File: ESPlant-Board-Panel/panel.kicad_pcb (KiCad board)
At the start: 2 copper layers, 156 x 147 mm, 408 parts, among them J1 Conn_01x05, U1 ESP32-C6-MINI-1/U, U3 Reset, U4 Boot, U5 Temp/Humid-Sensor, U6 Light sensor, U7 AMS1117-3_3, U8 MK-12C02-G025

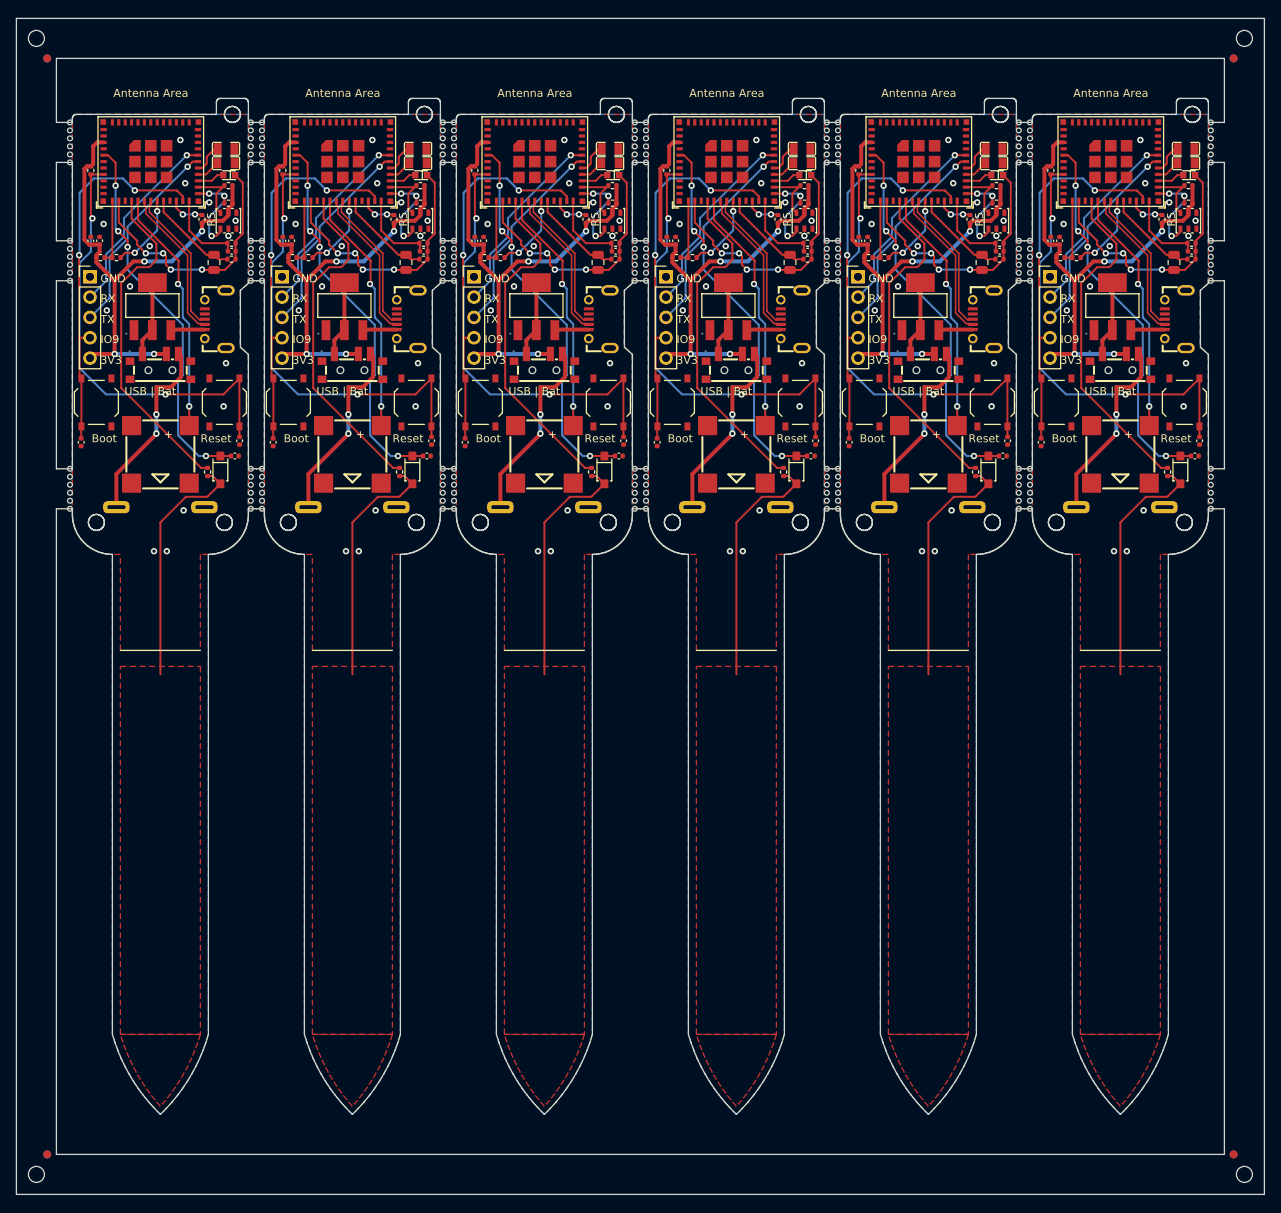
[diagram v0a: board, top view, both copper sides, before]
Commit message: Finish v2.0 for prototyping
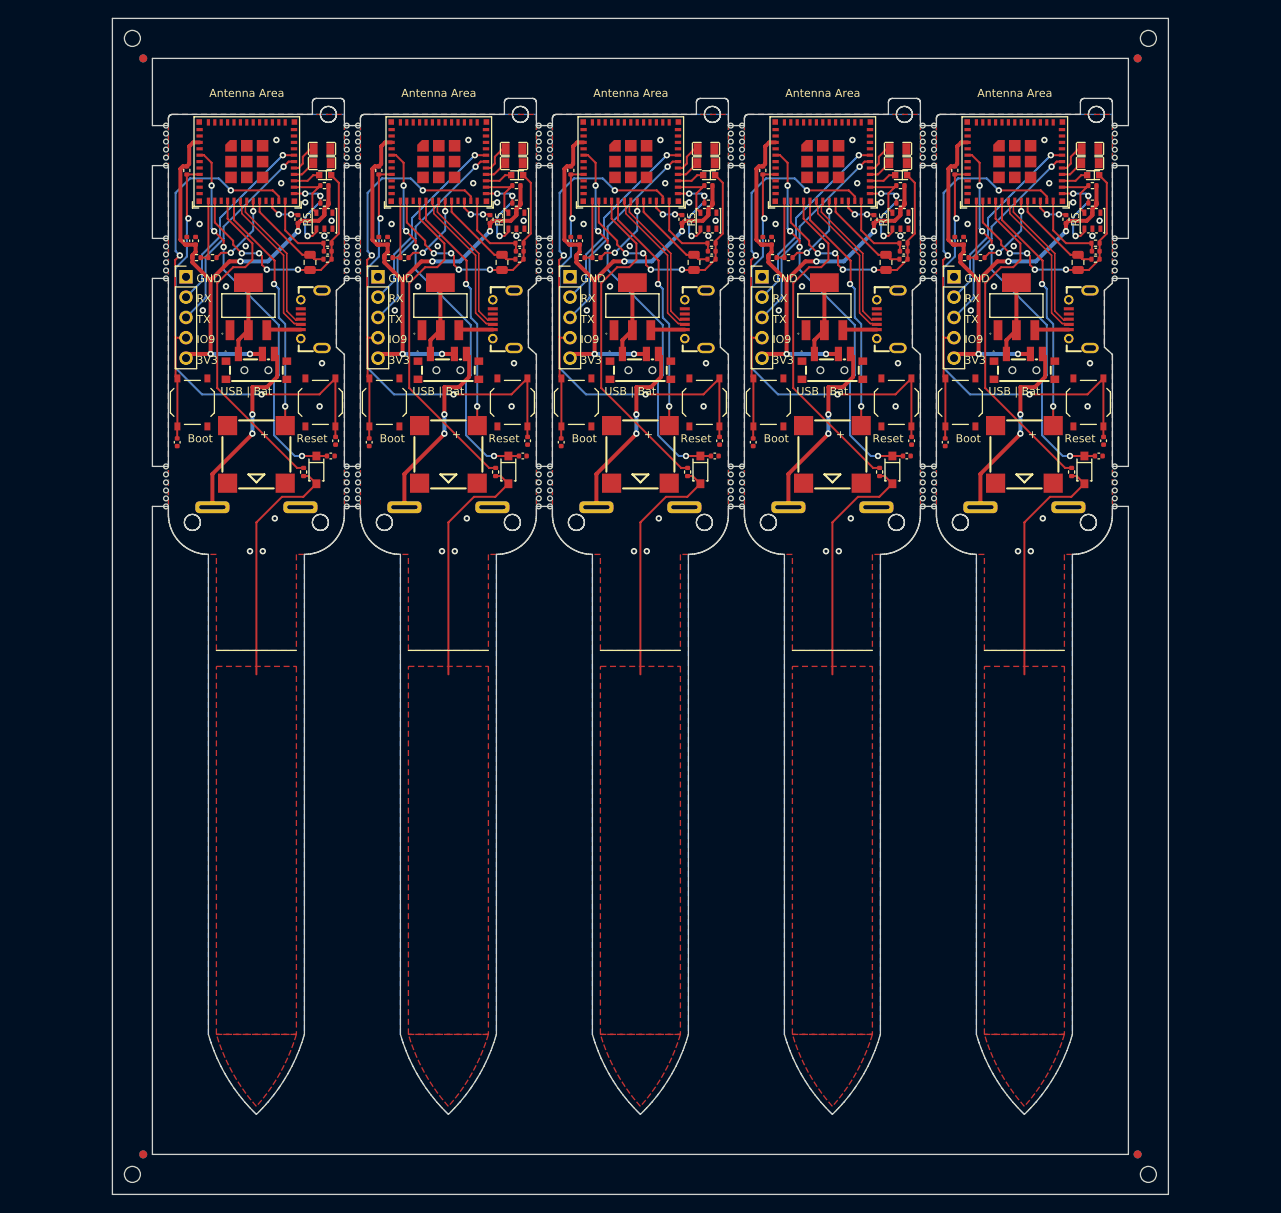
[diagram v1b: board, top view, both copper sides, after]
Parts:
- removed the BZ1 at (165.0, 74.5)
- removed the BZ1 at (237.0, 74.5)
- removed the BZ1 at (189.0, 74.5)
- removed the BZ1 at (213.0, 74.5)
- removed the BZ1 at (285.0, 74.5)
- removed the BZ1 at (261.0, 74.5)
- removed the C1 at (270.9, 72.8)
- removed the C1 at (198.9, 72.8)
- removed the C1 at (222.9, 72.8)
- removed the C1 at (246.9, 72.8)
- removed the C1 at (294.9, 72.8)
- removed the C1 at (174.9, 72.8)
- removed the C2 at (155.1, 73.0)
- removed the C2 at (251.1, 73.0)
- removed the C2 at (179.1, 73.0)
- removed the C2 at (275.1, 73.0)
- removed the C2 at (227.1, 73.0)
- removed the C2 at (203.1, 73.0)
- removed the C3 at (294.3, 74.7)
- removed the C3 at (222.3, 74.7)
- removed the C3 at (198.3, 74.7)
- removed the C3 at (246.3, 74.7)
- removed the C3 at (174.3, 74.7)
- removed the C3 at (270.3, 74.7)
- removed the C5 at (173.9, 49.1)
- removed the C5 at (269.9, 49.1)
- removed the C5 at (197.9, 49.1)
- removed the C5 at (293.9, 49.1)
- removed the C5 at (221.9, 49.1)
- removed the C5 at (245.9, 49.1)
- removed the C7 at (243.7, 50.5)
- removed the C7 at (219.7, 50.5)
- removed the C7 at (195.7, 50.5)
- removed the C7 at (267.7, 50.5)
- removed the C7 at (171.7, 50.5)
- removed the C7 at (291.7, 50.5)
- removed the C8 at (181.4, 47.8)
- removed the C8 at (229.4, 47.8)
- removed the C8 at (205.4, 47.8)
- removed the C8 at (253.4, 47.8)
- removed the C8 at (157.4, 47.8)
- removed the C8 at (277.4, 47.8)
- removed the C9 at (252.3, 47.8)
- removed the C9 at (204.3, 47.8)
- removed the C9 at (228.3, 47.8)
- removed the C9 at (156.3, 47.8)
- removed the C9 at (276.3, 47.8)
- removed the C9 at (180.3, 47.8)
- removed the D1 at (245.2, 36.3)
- removed the D1 at (293.2, 36.3)
- removed the D1 at (269.2, 36.3)
- removed the D1 at (221.2, 36.3)
- removed the D1 at (173.2, 36.3)
- removed the D1 at (197.2, 36.3)
- removed the D2 at (172.5, 76.4)
- removed the D2 at (220.5, 76.4)
- removed the D2 at (196.5, 76.4)
- removed the D2 at (292.5, 76.4)
- removed the D2 at (268.5, 76.4)
- removed the D2 at (244.5, 76.4)
- removed the D3 at (173.2, 38.1)
- removed the D3 at (197.2, 38.1)
- removed the D3 at (221.2, 38.1)
- removed the D3 at (245.2, 38.1)
- removed the D3 at (269.2, 38.1)
- removed the D3 at (293.2, 38.1)
- removed the J1 at (276.2, 52.3)
- removed the J1 at (204.2, 52.3)
- removed the J1 at (180.2, 52.3)
- removed the J1 at (228.2, 52.3)
- removed the J1 at (252.2, 52.3)
- removed the J1 at (156.2, 52.3)
- removed the R1 at (269.9, 48.1)
- removed the R1 at (173.9, 48.1)
- removed the R1 at (293.9, 48.1)
- removed the R1 at (221.9, 48.1)
- removed the R1 at (245.9, 48.1)
- removed the R1 at (197.9, 48.1)
- removed the R10 at (221.5, 43.1)
- removed the R10 at (245.5, 43.1)
- removed the R10 at (293.5, 43.1)
- removed the R10 at (197.5, 43.1)
- removed the R10 at (173.5, 43.1)
- removed the R10 at (269.5, 43.1)
- removed the R2 at (245.5, 40.9)
- removed the R2 at (221.5, 40.9)
- removed the R2 at (269.5, 40.9)
- removed the R2 at (293.5, 40.9)
- removed the R2 at (173.5, 40.9)
- removed the R2 at (197.5, 40.9)
- removed the R3 at (197.9, 50.1)
- removed the R3 at (173.9, 50.1)
- removed the R3 at (293.9, 50.1)
- removed the R3 at (245.9, 50.1)
- removed the R3 at (221.9, 50.1)
- removed the R3 at (269.9, 50.1)
- removed the R4 at (277.5, 49.9)
- removed the R4 at (205.5, 49.9)
- removed the R4 at (157.5, 49.9)
- removed the R4 at (181.5, 49.9)
- removed the R4 at (253.5, 49.9)
- removed the R4 at (229.5, 49.9)
- removed the R5 at (170.2, 45.1)
- removed the R5 at (266.2, 45.1)
- removed the R5 at (242.2, 45.1)
- removed the R5 at (194.2, 45.1)
- removed the R5 at (290.2, 45.1)
- removed the R5 at (218.2, 45.1)
- removed the R6 at (231.5, 49.9)
- removed the R6 at (183.5, 49.9)
- removed the R6 at (207.5, 49.9)
- removed the R6 at (255.5, 49.9)
- removed the R6 at (279.5, 49.9)
- removed the R6 at (159.5, 49.9)
- removed the R8 at (194.9, 76.7)
- removed the R8 at (266.9, 76.7)
- removed the R8 at (242.9, 76.7)
- removed the R8 at (290.9, 76.7)
- removed the R8 at (218.9, 76.7)
- removed the R8 at (170.9, 76.7)
- removed the R9 at (180.3, 39.0)
- removed the R9 at (252.3, 39.0)
- removed the R9 at (276.3, 39.0)
- removed the R9 at (204.3, 39.0)
- removed the R9 at (228.3, 39.0)
- removed the R9 at (156.3, 39.0)
- removed the REF** at (296.3, 34.0)
- removed the REF** at (224.3, 79.3)
- removed the REF** at (201.7, 50.8)
- removed the REF** at (249.7, 79.3)
- removed the REF** at (201.7, 79.3)
- removed the REF** at (200.3, 80.3)
- removed the REF** at (224.3, 51.8)
- removed the REF** at (153.7, 33.0)
- removed the REF** at (225.7, 50.8)
- removed the REF** at (200.3, 34.0)
- removed the REF** at (201.7, 52.8)
- removed the REF** at (176.3, 35.0)
- removed the REF** at (300.5, 164.5)
- removed the REF** at (201.7, 47.8)
- removed the REF** at (224.3, 50.8)
- removed the REF** at (272.3, 52.8)
- removed the REF** at (248.3, 48.8)
- removed the REF** at (248.3, 50.8)
- removed the REF** at (248.3, 36.0)
- removed the REF** at (176.3, 36.0)
- removed the REF** at (296.3, 52.8)
- removed the REF** at (273.7, 80.3)
- removed the REF** at (153.7, 80.3)
- removed the REF** at (225.7, 38.0)
- removed the REF** at (249.7, 36.0)
- removed the REF** at (177.7, 36.0)
- removed the REF** at (150.9, 25.0) (x2)
- removed the REF** at (177.7, 81.3)
- removed the REF** at (249.7, 48.8)
- removed the REF** at (224.3, 33.0)
- removed the REF** at (153.7, 35.0)
- removed the REF** at (272.3, 35.0)
- removed the REF** at (201.7, 36.0)
- removed the REF** at (225.7, 78.3)
- removed the REF** at (272.3, 38.0)
- removed the REF** at (224.3, 34.0)
- removed the REF** at (153.7, 52.8)
- removed the REF** at (200.3, 77.3)
- removed the REF** at (177.7, 76.3)
- removed the REF** at (201.7, 80.3)
- removed the REF** at (224.3, 35.0)
- removed the REF** at (225.7, 76.3)
- removed the REF** at (225.7, 79.3)
- removed the REF** at (225.7, 77.3)
- removed the REF** at (225.7, 48.8)
- removed the REF** at (150.9, 162.0) (x2)
- removed the REF** at (272.3, 49.8)
- removed the REF** at (296.3, 81.3)
- removed the REF** at (248.3, 79.3)
- removed the REF** at (299.2, 162.0) (x2)
- removed the REF** at (249.7, 34.0)
- removed the REF** at (200.3, 49.8)
- removed the REF** at (273.7, 47.8)
- removed the REF** at (200.3, 38.0)
- removed the REF** at (200.3, 52.8)
- removed the REF** at (272.3, 48.8)
- removed the REF** at (176.3, 79.3)
- removed the REF** at (149.5, 164.5)
- removed the REF** at (273.7, 37.0)
- removed the REF** at (273.7, 81.3)
- removed the REF** at (225.7, 34.0)
- removed the REF** at (248.3, 78.3)
- removed the REF** at (249.7, 37.0)
- removed the REF** at (153.7, 76.3)
- removed the REF** at (201.7, 35.0)
- removed the REF** at (153.7, 47.8)
- removed the REF** at (296.3, 38.0)
- removed the REF** at (296.3, 78.3)
- removed the REF** at (176.3, 33.0)
- removed the REF** at (176.3, 37.0)
- removed the REF** at (248.3, 49.8)
- removed the REF** at (249.7, 50.8)
- removed the REF** at (272.3, 76.3)
- removed the REF** at (200.3, 36.0)
- removed the REF** at (273.7, 33.0)
- removed the REF** at (273.7, 78.3)
- removed the REF** at (248.3, 81.3)
- removed the REF** at (248.3, 35.0)
- removed the REF** at (224.3, 49.8)
- removed the REF** at (225.7, 36.0)
- removed the REF** at (296.3, 47.8)
- removed the REF** at (153.7, 81.3)
- removed the REF** at (176.3, 38.0)
- removed the REF** at (177.7, 34.0)
- removed the REF** at (249.7, 47.8)
- removed the REF** at (225.7, 47.8)
- removed the REF** at (153.7, 34.0)
- removed the REF** at (177.7, 37.0)
- removed the REF** at (200.3, 48.8)
- removed the REF** at (225.7, 52.8)
- removed the REF** at (296.3, 49.8)
- removed the REF** at (248.3, 37.0)
- removed the REF** at (296.3, 76.3)
- removed the REF** at (273.7, 35.0)
- removed the REF** at (201.7, 38.0)
- removed the REF** at (201.7, 48.8)
- removed the REF** at (248.3, 38.0)
- removed the REF** at (176.3, 77.3)
- removed the REF** at (224.3, 78.3)
- removed the REF** at (177.7, 35.0)
- removed the REF** at (224.3, 47.8)
- removed the REF** at (176.3, 51.8)
- removed the REF** at (273.7, 52.8)
- removed the REF** at (153.7, 50.8)
- removed the REF** at (248.3, 47.8)
- removed the REF** at (201.7, 51.8)
- removed the REF** at (272.3, 80.3)
- removed the REF** at (153.7, 48.8)
- removed the REF** at (153.7, 38.0)
- removed the REF** at (299.2, 25.0) (x2)
- removed the REF** at (296.3, 80.3)
- removed the REF** at (225.7, 33.0)
- removed the REF** at (273.7, 34.0)
- removed the REF** at (177.7, 50.8)
- removed the REF** at (176.3, 50.8)
- removed the REF** at (273.7, 36.0)
- removed the REF** at (153.7, 36.0)
- removed the REF** at (249.7, 80.3)
- removed the REF** at (176.3, 48.8)
- removed the REF** at (200.3, 76.3)
- removed the REF** at (273.7, 79.3)
- removed the REF** at (248.3, 80.3)
- removed the REF** at (153.7, 79.3)
- removed the REF** at (176.3, 78.3)
- removed the REF** at (296.3, 77.3)
- removed the REF** at (249.7, 76.3)
- removed the REF** at (177.7, 47.8)
- removed the REF** at (177.7, 33.0)
- removed the REF** at (224.3, 37.0)
- removed the REF** at (248.3, 33.0)
- removed the REF** at (200.3, 78.3)
- removed the REF** at (272.3, 81.3)
- removed the REF** at (296.3, 50.8)
- removed the REF** at (153.7, 37.0)
- removed the REF** at (225.7, 49.8)
- removed the REF** at (248.3, 34.0)
- removed the REF** at (225.7, 51.8)
- removed the REF** at (272.3, 77.3)
- removed the REF** at (248.3, 52.8)
- removed the REF** at (201.7, 76.3)
- removed the REF** at (177.7, 80.3)
- removed the REF** at (201.7, 81.3)
- removed the REF** at (153.7, 51.8)
- removed the REF** at (296.3, 48.8)
- removed the REF** at (149.5, 22.5)
- removed the REF** at (177.7, 49.8)
- removed the REF** at (200.3, 35.0)
- removed the REF** at (273.7, 76.3)
- removed the REF** at (201.7, 49.8)
- removed the REF** at (249.7, 77.3)
- removed the REF** at (272.3, 37.0)
- removed the REF** at (249.7, 35.0)
- removed the REF** at (248.3, 77.3)
- removed the REF** at (201.7, 37.0)
- removed the REF** at (273.7, 50.8)
- removed the REF** at (177.7, 52.8)
- removed the REF** at (249.7, 78.3)
- removed the REF** at (296.3, 79.3)
- removed the REF** at (224.3, 36.0)
- removed the REF** at (153.7, 78.3)
- removed the REF** at (296.3, 51.8)
- removed the REF** at (249.7, 49.8)
- removed the REF** at (200.3, 79.3)
- removed the REF** at (176.3, 34.0)
- removed the REF** at (201.7, 33.0)
- removed the REF** at (248.3, 51.8)
- removed the REF** at (224.3, 48.8)
- removed the REF** at (272.3, 51.8)
- removed the REF** at (296.3, 33.0)
- removed the REF** at (177.7, 77.3)
- removed the REF** at (272.3, 78.3)
- removed the REF** at (200.3, 33.0)
- removed the REF** at (300.5, 22.5)
- removed the REF** at (176.3, 81.3)
- removed the REF** at (225.7, 35.0)
- removed the REF** at (225.7, 80.3)
- removed the REF** at (224.3, 81.3)
- removed the REF** at (224.3, 77.3)
- removed the REF** at (153.7, 77.3)
- removed the REF** at (177.7, 78.3)
- removed the REF** at (177.7, 51.8)
- removed the REF** at (272.3, 36.0)
- removed the REF** at (249.7, 38.0)
- removed the REF** at (225.7, 37.0)
- removed the REF** at (200.3, 81.3)
- removed the REF** at (296.3, 35.0)
- removed the REF** at (200.3, 51.8)
- removed the REF** at (176.3, 80.3)
- removed the REF** at (201.7, 34.0)
- removed the REF** at (249.7, 81.3)
- removed the REF** at (272.3, 33.0)
- removed the REF** at (272.3, 79.3)
- removed the REF** at (273.7, 77.3)
- removed the REF** at (272.3, 34.0)
- removed the REF** at (224.3, 76.3)
- removed the REF** at (176.3, 76.3)
- removed the REF** at (201.7, 77.3)
- removed the REF** at (176.3, 47.8)
- removed the REF** at (272.3, 47.8)
- removed the REF** at (224.3, 80.3)
- removed the REF** at (177.7, 38.0)
- removed the REF** at (249.7, 52.8)
- removed the REF** at (177.7, 79.3)
- removed the REF** at (200.3, 47.8)
- removed the REF** at (224.3, 38.0)
- removed the REF** at (273.7, 38.0)
- removed the REF** at (249.7, 33.0)
- removed the REF** at (296.3, 37.0)
- removed the REF** at (224.3, 52.8)
- removed the REF** at (273.7, 49.8)
- removed the REF** at (200.3, 50.8)
- removed the REF** at (177.7, 48.8)
- removed the REF** at (176.3, 52.8)
- removed the REF** at (200.3, 37.0)
- removed the REF** at (273.7, 51.8)
- removed the REF** at (225.7, 81.3)
- removed the REF** at (201.7, 78.3)
- removed the REF** at (273.7, 48.8)
- removed the REF** at (176.3, 49.8)
- removed the REF** at (296.3, 36.0)
- removed the REF** at (153.7, 49.8)
- removed the REF** at (272.3, 50.8)
- removed the REF** at (249.7, 51.8)
- removed the REF** at (248.3, 76.3)
- removed the U1 at (211.8, 35.2)
- removed the U1 at (235.8, 35.2)
- removed the U1 at (259.8, 35.2)
- removed the U1 at (283.8, 35.2)
- removed the U1 at (187.8, 35.2)
- removed the U1 at (163.8, 35.2)
- removed the U3 at (269.0, 68.0)
- removed the U3 at (221.0, 68.0)
- removed the U3 at (245.0, 68.0)
- removed the U3 at (293.0, 68.0)
- removed the U3 at (173.0, 68.0)
- removed the U3 at (197.0, 68.0)
- removed the U4 at (181.0, 68.0)
- removed the U4 at (229.0, 68.0)
- removed the U4 at (277.0, 68.0)
- removed the U4 at (205.0, 68.0)
- removed the U4 at (157.0, 68.0)
- removed the U4 at (253.0, 68.0)
- removed the U5 at (269.5, 45.3)
- removed the U5 at (293.5, 45.3)
- removed the U5 at (173.5, 45.3)
- removed the U5 at (221.5, 45.3)
- removed the U5 at (245.5, 45.3)
- removed the U5 at (197.5, 45.3)
- removed the U6 at (245.6, 39.6)
- removed the U6 at (221.6, 39.6)
- removed the U6 at (173.6, 39.6)
- removed the U6 at (293.6, 39.6)
- removed the U6 at (269.6, 39.6)
- removed the U6 at (197.6, 39.6)
- removed the U7 at (188.0, 56.0)
- removed the U7 at (164.0, 56.0)
- removed the U7 at (236.0, 56.0)
- removed the U7 at (212.0, 56.0)
- removed the U7 at (260.0, 56.0)
- removed the U7 at (284.0, 56.0)
- removed the U8 at (285.0, 63.5)
- removed the U8 at (237.0, 63.5)
- removed the U8 at (261.0, 63.5)
- removed the U8 at (165.0, 63.5)
- removed the U8 at (213.0, 63.5)
- removed the U8 at (189.0, 63.5)
- removed the U9 at (165.0, 81.1)
- removed the U9 at (285.0, 81.1)
- removed the U9 at (213.0, 81.1)
- removed the U9 at (261.0, 81.1)
- removed the U9 at (189.0, 81.1)
- removed the U9 at (237.0, 81.1)
- removed the USB1 at (195.9, 57.6)
- removed the USB1 at (267.9, 57.6)
- removed the USB1 at (219.9, 57.6)
- removed the USB1 at (171.9, 57.6)
- removed the USB1 at (243.9, 57.6)
- removed the USB1 at (291.9, 57.6)
- added BZ1: Buzzer, CustomFootprints:BUZ-SMD_4P-L8.5-W8.5-P8.50-BR, F.Cu at (249.0, 74.5)
- added BZ1: Buzzer, CustomFootprints:BUZ-SMD_4P-L8.5-W8.5-P8.50-BR, F.Cu at (201.0, 74.5)
- added BZ1: Buzzer, CustomFootprints:BUZ-SMD_4P-L8.5-W8.5-P8.50-BR, F.Cu at (177.0, 74.5)
- added BZ1: Buzzer, CustomFootprints:BUZ-SMD_4P-L8.5-W8.5-P8.50-BR, F.Cu at (273.0, 74.5)
- added BZ1: Buzzer, CustomFootprints:BUZ-SMD_4P-L8.5-W8.5-P8.50-BR, F.Cu at (225.0, 74.5)
- added C1: 100nF, Capacitor_SMD:C_0402_1005Metric, F.Cu at (186.9, 72.8)
- added C1: 100nF, Capacitor_SMD:C_0402_1005Metric, F.Cu at (210.9, 72.8)
- added C1: 100nF, Capacitor_SMD:C_0402_1005Metric, F.Cu at (258.9, 72.8)
- added C1: 100nF, Capacitor_SMD:C_0402_1005Metric, F.Cu at (234.9, 72.8)
- added C1: 100nF, Capacitor_SMD:C_0402_1005Metric, F.Cu at (282.9, 72.8)
- added C2: 100nF, Capacitor_SMD:C_0402_1005Metric, F.Cu at (263.1, 73.0)
- added C2: 100nF, Capacitor_SMD:C_0402_1005Metric, F.Cu at (239.1, 73.0)
- added C2: 100nF, Capacitor_SMD:C_0402_1005Metric, F.Cu at (215.1, 73.0)
- added C2: 100nF, Capacitor_SMD:C_0402_1005Metric, F.Cu at (167.1, 73.0)
- added C2: 100nF, Capacitor_SMD:C_0402_1005Metric, F.Cu at (191.1, 73.0)
- added C3: 150pF, Capacitor_SMD:C_0402_1005Metric, F.Cu at (210.3, 74.7)
- added C3: 150pF, Capacitor_SMD:C_0402_1005Metric, F.Cu at (258.3, 74.7)
- added C3: 150pF, Capacitor_SMD:C_0402_1005Metric, F.Cu at (186.3, 74.7)
- added C3: 150pF, Capacitor_SMD:C_0402_1005Metric, F.Cu at (234.3, 74.7)
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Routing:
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- removed copper zone on F.Cu, net Board_5-/SensorCapV
- removed copper zone on B.Cu, net Board_5-GND
- removed copper zone on F.Cu, net Board_5-GND
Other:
- board size 156 x 147 mm -> 132 x 147 mm

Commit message: Board: Update panel
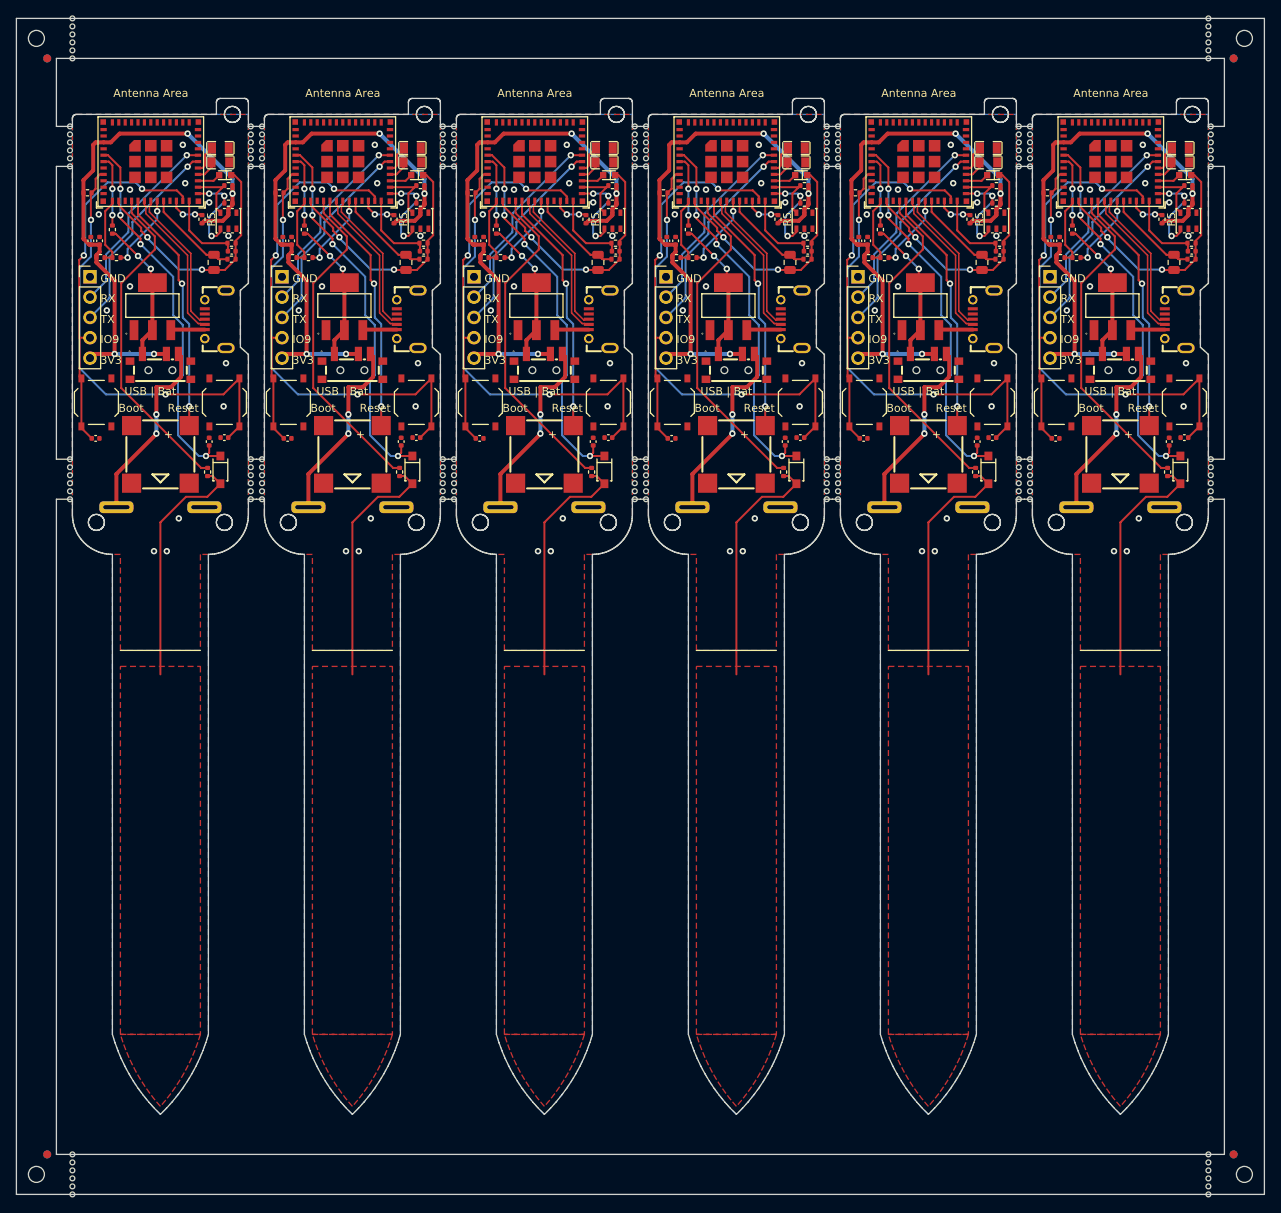
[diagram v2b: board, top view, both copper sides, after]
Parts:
- removed the BZ1 at (249.0, 74.5)
- removed the BZ1 at (201.0, 74.5)
- removed the BZ1 at (177.0, 74.5)
- removed the BZ1 at (273.0, 74.5)
- removed the BZ1 at (225.0, 74.5)
- removed the C1 at (186.9, 72.8)
- removed the C1 at (210.9, 72.8)
- removed the C1 at (258.9, 72.8)
- removed the C1 at (234.9, 72.8)
- removed the C1 at (282.9, 72.8)
- removed the C2 at (263.1, 73.0)
- removed the C2 at (239.1, 73.0)
- removed the C2 at (215.1, 73.0)
- removed the C2 at (167.1, 73.0)
- removed the C2 at (191.1, 73.0)
- removed the C3 at (210.3, 74.7)
- removed the C3 at (258.3, 74.7)
- removed the C3 at (186.3, 74.7)
- removed the C3 at (234.3, 74.7)
- removed the C3 at (282.3, 74.7)
- removed the C5 at (185.9, 49.1)
- removed the C5 at (257.9, 49.1)
- removed the C5 at (281.9, 49.1)
- removed the C5 at (233.9, 49.1)
- removed the C5 at (209.9, 49.1)
- removed the C7 at (231.7, 50.5)
- removed the C7 at (255.7, 50.5)
- removed the C7 at (183.7, 50.5)
- removed the C7 at (279.7, 50.5)
- removed the C7 at (207.7, 50.5)
- removed the C8 at (193.4, 47.8)
- removed the C8 at (241.4, 47.8)
- removed the C8 at (265.4, 47.8)
- removed the C8 at (217.4, 47.8)
- removed the C8 at (169.4, 47.8)
- removed the C9 at (168.3, 47.8)
- removed the C9 at (264.3, 47.8)
- removed the C9 at (216.3, 47.8)
- removed the C9 at (192.3, 47.8)
- removed the C9 at (240.3, 47.8)
- removed the D1 at (281.2, 36.3)
- removed the D1 at (233.2, 36.3)
- removed the D1 at (209.2, 36.3)
- removed the D1 at (185.2, 36.3)
- removed the D1 at (257.2, 36.3)
- removed the D2 at (232.5, 76.4)
- removed the D2 at (184.5, 76.4)
- removed the D2 at (280.5, 76.4)
- removed the D2 at (256.5, 76.4)
- removed the D2 at (208.5, 76.4)
- removed the D3 at (257.2, 38.1)
- removed the D3 at (209.2, 38.1)
- removed the D3 at (281.2, 38.1)
- removed the D3 at (233.2, 38.1)
- removed the D3 at (185.2, 38.1)
- removed the J1 at (168.2, 52.3)
- removed the J1 at (216.2, 52.3)
- removed the J1 at (264.2, 52.3)
- removed the J1 at (240.2, 52.3)
- removed the J1 at (192.2, 52.3)
- removed the R1 at (185.9, 48.1)
- removed the R1 at (209.9, 48.1)
- removed the R1 at (281.9, 48.1)
- removed the R1 at (257.9, 48.1)
- removed the R1 at (233.9, 48.1)
- removed the R10 at (209.5, 43.1)
- removed the R10 at (257.5, 43.1)
- removed the R10 at (233.5, 43.1)
- removed the R10 at (281.5, 43.1)
- removed the R10 at (185.5, 43.1)
- removed the R2 at (281.5, 40.9)
- removed the R2 at (257.5, 40.9)
- removed the R2 at (209.5, 40.9)
- removed the R2 at (185.5, 40.9)
- removed the R2 at (233.5, 40.9)
- removed the R3 at (185.9, 50.1)
- removed the R3 at (257.9, 50.1)
- removed the R3 at (233.9, 50.1)
- removed the R3 at (209.9, 50.1)
- removed the R3 at (281.9, 50.1)
- removed the R4 at (193.5, 49.9)
- removed the R4 at (169.5, 49.9)
- removed the R4 at (241.5, 49.9)
- removed the R4 at (265.5, 49.9)
- removed the R4 at (217.5, 49.9)
- removed the R5 at (278.2, 45.1)
- removed the R5 at (254.2, 45.1)
- removed the R5 at (230.2, 45.1)
- removed the R5 at (206.2, 45.1)
- removed the R5 at (182.2, 45.1)
- removed the R6 at (195.5, 49.9)
- removed the R6 at (219.5, 49.9)
- removed the R6 at (171.5, 49.9)
- removed the R6 at (267.5, 49.9)
- removed the R6 at (243.5, 49.9)
- removed the R8 at (254.9, 76.7)
- removed the R8 at (206.9, 76.7)
- removed the R8 at (182.9, 76.7)
- removed the R8 at (278.9, 76.7)
- removed the R8 at (230.9, 76.7)
- removed the R9 at (264.3, 39.0)
- removed the R9 at (216.3, 39.0)
- removed the R9 at (192.3, 39.0)
- removed the R9 at (168.3, 39.0)
- removed the R9 at (240.3, 39.0)
- removed the REF** at (260.3, 81.0)
- removed the REF** at (188.3, 51.5)
- removed the REF** at (236.3, 48.5)
- removed the REF** at (260.3, 52.5)
- removed the REF** at (213.7, 50.5)
- removed the REF** at (236.3, 37.4)
- removed the REF** at (260.3, 76.0)
- removed the REF** at (165.7, 37.4)
- removed the REF** at (260.3, 49.5)
- removed the REF** at (284.3, 77.0)
- removed the REF** at (260.3, 80.0)
- removed the REF** at (161.5, 22.5)
- removed the REF** at (288.5, 164.5)
- removed the REF** at (212.3, 48.5)
- removed the REF** at (260.3, 36.4)
- removed the REF** at (261.7, 79.0)
- removed the REF** at (237.7, 50.5)
- removed the REF** at (236.3, 33.4)
- removed the REF** at (260.3, 35.4)
- removed the REF** at (261.7, 33.4)
- removed the REF** at (237.7, 47.5)
- removed the REF** at (212.3, 52.5)
- removed the REF** at (165.7, 35.4)
- removed the REF** at (261.7, 77.0)
- removed the REF** at (188.3, 34.4)
- removed the REF** at (212.3, 49.5)
- removed the REF** at (260.3, 77.0)
- removed the REF** at (189.7, 34.4)
- removed the REF** at (261.7, 80.0)
- removed the REF** at (189.7, 78.0)
- removed the REF** at (213.7, 52.5)
- removed the REF** at (260.3, 37.4)
- removed the REF** at (260.3, 47.5)
- removed the REF** at (189.7, 48.5)
- removed the REF** at (189.7, 76.0)
- removed the REF** at (236.3, 78.0)
- removed the REF** at (165.7, 51.5)
- removed the REF** at (188.3, 33.4)
- removed the REF** at (261.7, 37.4)
- removed the REF** at (261.7, 36.4)
- removed the REF** at (189.7, 35.4)
- removed the REF** at (237.7, 51.5)
- removed the REF** at (236.3, 47.5)
- removed the REF** at (261.7, 78.0)
- removed the REF** at (284.3, 79.0)
- removed the REF** at (236.3, 36.4)
- removed the REF** at (236.3, 81.0)
- removed the REF** at (236.3, 50.5)
- removed the REF** at (236.3, 79.0)
- removed the REF** at (165.7, 78.0)
- removed the REF** at (213.7, 51.5)
- removed the REF** at (261.7, 47.5)
- removed the REF** at (236.3, 52.5)
- removed the REF** at (261.7, 38.4)
- removed the REF** at (189.7, 33.4)
- removed the REF** at (213.7, 37.4)
- removed the REF** at (189.7, 37.4)
- removed the REF** at (188.3, 80.0)
- removed the REF** at (236.3, 77.0)
- removed the REF** at (213.7, 81.0)
- removed the REF** at (213.7, 36.4)
- removed the REF** at (261.7, 51.5)
- removed the REF** at (212.3, 38.4)
- removed the REF** at (237.7, 34.4)
- removed the REF** at (236.3, 38.4)
- removed the REF** at (261.7, 81.0)
- removed the REF** at (188.3, 52.5)
- removed the REF** at (237.7, 48.5)
- removed the REF** at (189.7, 52.5)
- removed the REF** at (165.7, 36.4)
- removed the REF** at (165.7, 52.5)
- removed the REF** at (237.7, 49.5)
- removed the REF** at (189.7, 79.0)
- removed the REF** at (165.7, 48.5)
- removed the REF** at (261.7, 49.5)
- removed the REF** at (188.3, 38.4)
- removed the REF** at (188.3, 49.5)
- removed the REF** at (213.7, 78.0)
- removed the REF** at (284.3, 36.4)
- removed the REF** at (162.9, 162.0) (x2)
- removed the REF** at (212.3, 37.4)
- removed the REF** at (284.3, 49.5)
- removed the REF** at (165.7, 50.5)
- removed the REF** at (237.7, 79.0)
- removed the REF** at (161.5, 164.5)
- removed the REF** at (284.3, 50.5)
- removed the REF** at (260.3, 51.5)
- removed the REF** at (284.3, 38.4)
- removed the REF** at (165.7, 79.0)
- removed the REF** at (261.7, 50.5)
- removed the REF** at (189.7, 49.5)
- removed the REF** at (189.7, 77.0)
- removed the REF** at (212.3, 50.5)
- removed the REF** at (165.7, 34.4)
- removed the REF** at (213.7, 49.5)
- removed the REF** at (213.7, 80.0)
- removed the REF** at (165.7, 76.0)
- removed the REF** at (189.7, 80.0)
- removed the REF** at (212.3, 36.4)
- removed the REF** at (287.2, 162.0) (x2)
- removed the REF** at (189.7, 50.5)
- removed the REF** at (287.2, 25.0) (x2)
- removed the REF** at (162.9, 25.0) (x2)
- removed the REF** at (188.3, 37.4)
- removed the REF** at (260.3, 50.5)
- removed the REF** at (288.5, 22.5)
- removed the REF** at (260.3, 38.4)
- removed the REF** at (212.3, 81.0)
- removed the REF** at (237.7, 38.4)
- removed the REF** at (284.3, 37.4)
- removed the REF** at (188.3, 81.0)
- removed the REF** at (165.7, 77.0)
- removed the REF** at (237.7, 76.0)
- removed the REF** at (284.3, 78.0)
- removed the REF** at (261.7, 52.5)
- removed the REF** at (212.3, 33.4)
- removed the REF** at (189.7, 47.5)
- removed the REF** at (165.7, 80.0)
- removed the REF** at (260.3, 48.5)
- removed the REF** at (284.3, 48.5)
- removed the REF** at (213.7, 34.4)
- removed the REF** at (284.3, 35.4)
- removed the REF** at (284.3, 81.0)
- removed the REF** at (165.7, 47.5)
- removed the REF** at (261.7, 34.4)
- removed the REF** at (236.3, 35.4)
- removed the REF** at (236.3, 76.0)
- removed the REF** at (237.7, 77.0)
- removed the REF** at (189.7, 51.5)
- removed the REF** at (261.7, 35.4)
- removed the REF** at (189.7, 81.0)
- removed the REF** at (213.7, 77.0)
- removed the REF** at (212.3, 79.0)
- removed the REF** at (237.7, 81.0)
- removed the REF** at (236.3, 49.5)
- removed the REF** at (188.3, 36.4)
- removed the REF** at (188.3, 35.4)
- removed the REF** at (284.3, 80.0)
- removed the REF** at (237.7, 78.0)
- removed the REF** at (188.3, 78.0)
- removed the REF** at (188.3, 77.0)
- removed the REF** at (213.7, 35.4)
- removed the REF** at (236.3, 51.5)
- removed the REF** at (261.7, 76.0)
- removed the REF** at (213.7, 79.0)
- removed the REF** at (212.3, 77.0)
- removed the REF** at (237.7, 35.4)
- removed the REF** at (237.7, 33.4)
- removed the REF** at (261.7, 48.5)
- removed the REF** at (284.3, 33.4)
- removed the REF** at (212.3, 47.5)
- removed the REF** at (165.7, 49.5)
- removed the REF** at (212.3, 78.0)
- removed the REF** at (260.3, 78.0)
- removed the REF** at (188.3, 79.0)
- removed the REF** at (260.3, 79.0)
- removed the REF** at (236.3, 34.4)
- removed the REF** at (236.3, 80.0)
- removed the REF** at (212.3, 35.4)
- removed the REF** at (189.7, 36.4)
- removed the REF** at (237.7, 52.5)
- removed the REF** at (284.3, 76.0)
- removed the REF** at (213.7, 47.5)
- removed the REF** at (212.3, 76.0)
- removed the REF** at (212.3, 80.0)
- removed the REF** at (284.3, 52.5)
- removed the REF** at (165.7, 33.4)
- removed the REF** at (284.3, 51.5)
- removed the REF** at (260.3, 33.4)
- removed the REF** at (165.7, 38.4)
- removed the REF** at (284.3, 47.5)
- removed the REF** at (188.3, 48.5)
- removed the REF** at (188.3, 76.0)
- removed the REF** at (237.7, 36.4)
- removed the REF** at (212.3, 34.4)
- removed the REF** at (213.7, 48.5)
- removed the REF** at (213.7, 38.4)
- removed the REF** at (188.3, 47.5)
- removed the REF** at (189.7, 38.4)
- removed the REF** at (165.7, 81.0)
- removed the REF** at (237.7, 80.0)
- removed the REF** at (213.7, 76.0)
- removed the REF** at (284.3, 34.4)
- removed the REF** at (188.3, 50.5)
- removed the REF** at (212.3, 51.5)
- removed the REF** at (237.7, 37.4)
- removed the REF** at (213.7, 33.4)
- removed the REF** at (260.3, 34.4)
- removed the U1 at (199.8, 35.2)
- removed the U1 at (247.8, 35.2)
- removed the U1 at (223.8, 35.2)
- removed the U1 at (175.8, 35.2)
- removed the U1 at (271.8, 35.2)
- removed the U3 at (185.0, 68.0)
- removed the U3 at (281.0, 68.0)
- removed the U3 at (209.0, 68.0)
- removed the U3 at (233.0, 68.0)
- removed the U3 at (257.0, 68.0)
- removed the U4 at (265.0, 68.0)
- removed the U4 at (169.0, 68.0)
- removed the U4 at (193.0, 68.0)
- removed the U4 at (217.0, 68.0)
- removed the U4 at (241.0, 68.0)
- removed the U5 at (257.5, 45.3)
- removed the U5 at (281.5, 45.3)
- removed the U5 at (233.5, 45.3)
- removed the U5 at (209.5, 45.3)
- removed the U5 at (185.5, 45.3)
- removed the U6 at (281.6, 39.6)
- removed the U6 at (209.6, 39.6)
- removed the U6 at (233.6, 39.6)
- removed the U6 at (257.6, 39.6)
- removed the U6 at (185.6, 39.6)
- removed the U7 at (200.0, 56.0)
- removed the U7 at (272.0, 56.0)
- removed the U7 at (248.0, 56.0)
- removed the U7 at (176.0, 56.0)
- removed the U7 at (224.0, 56.0)
- removed the U8 at (201.0, 63.5)
- removed the U8 at (273.0, 63.5)
- removed the U8 at (177.0, 63.5)
- removed the U8 at (225.0, 63.5)
- removed the U8 at (249.0, 63.5)
- removed the U9 at (273.0, 81.1)
- removed the U9 at (177.0, 81.1)
- removed the U9 at (249.0, 81.1)
- removed the U9 at (225.0, 81.1)
- removed the U9 at (201.0, 81.1)
- removed the USB1 at (183.9, 57.6)
- removed the USB1 at (231.9, 57.6)
- removed the USB1 at (255.9, 57.6)
- removed the USB1 at (207.9, 57.6)
- removed the USB1 at (279.9, 57.6)
- added BZ1: Buzzer, CustomFootprints:BUZ-SMD_4P-L8.5-W8.5-P8.50-BR, F.Cu at (285.0, 74.5)
- added BZ1: Buzzer, CustomFootprints:BUZ-SMD_4P-L8.5-W8.5-P8.50-BR, F.Cu at (213.0, 74.5)
- added BZ1: Buzzer, CustomFootprints:BUZ-SMD_4P-L8.5-W8.5-P8.50-BR, F.Cu at (237.0, 74.5)
- added BZ1: Buzzer, CustomFootprints:BUZ-SMD_4P-L8.5-W8.5-P8.50-BR, F.Cu at (189.0, 74.5)
- added BZ1: Buzzer, CustomFootprints:BUZ-SMD_4P-L8.5-W8.5-P8.50-BR, F.Cu at (165.0, 74.5)
- added BZ1: Buzzer, CustomFootprints:BUZ-SMD_4P-L8.5-W8.5-P8.50-BR, F.Cu at (261.0, 74.5)
- added C1: 100nF, Capacitor_SMD:C_0402_1005Metric, F.Cu at (197.0, 72.4)
- added C1: 100nF, Capacitor_SMD:C_0402_1005Metric, F.Cu at (293.0, 72.4)
- added C1: 100nF, Capacitor_SMD:C_0402_1005Metric, F.Cu at (221.0, 72.4)
- added C1: 100nF, Capacitor_SMD:C_0402_1005Metric, F.Cu at (173.0, 72.4)
- added C1: 100nF, Capacitor_SMD:C_0402_1005Metric, F.Cu at (269.0, 72.4)
- added C1: 100nF, Capacitor_SMD:C_0402_1005Metric, F.Cu at (245.0, 72.4)
- added C2: 100nF, Capacitor_SMD:C_0402_1005Metric, F.Cu at (204.9, 72.5)
- added C2: 100nF, Capacitor_SMD:C_0402_1005Metric, F.Cu at (276.9, 72.5)
- added C2: 100nF, Capacitor_SMD:C_0402_1005Metric, F.Cu at (252.9, 72.5)
- added C2: 100nF, Capacitor_SMD:C_0402_1005Metric, F.Cu at (228.9, 72.5)
- added C2: 100nF, Capacitor_SMD:C_0402_1005Metric, F.Cu at (180.9, 72.5)
- added C2: 100nF, Capacitor_SMD:C_0402_1005Metric, F.Cu at (156.9, 72.5)
- added C3: 150pF, Capacitor_SMD:C_0402_1005Metric, F.Cu at (267.1, 72.9)
- added C3: 150pF, Capacitor_SMD:C_0402_1005Metric, F.Cu at (291.1, 72.9)
- added C3: 150pF, Capacitor_SMD:C_0402_1005Metric, F.Cu at (243.1, 72.9)
- added C3: 150pF, Capacitor_SMD:C_0402_1005Metric, F.Cu at (219.1, 72.9)
- added C3: 150pF, Capacitor_SMD:C_0402_1005Metric, F.Cu at (195.1, 72.9)
- added C3: 150pF, Capacitor_SMD:C_0402_1005Metric, F.Cu at (171.1, 72.9)
- added C5: 100nF, Capacitor_SMD:C_0402_1005Metric, F.Cu at (269.9, 49.1)
- added C5: 100nF, Capacitor_SMD:C_0402_1005Metric, F.Cu at (293.9, 49.1)
- added C5: 100nF, Capacitor_SMD:C_0402_1005Metric, F.Cu at (197.9, 49.1)
- added C5: 100nF, Capacitor_SMD:C_0402_1005Metric, F.Cu at (173.9, 49.1)
- added C5: 100nF, Capacitor_SMD:C_0402_1005Metric, F.Cu at (221.9, 49.1)
- added C5: 100nF, Capacitor_SMD:C_0402_1005Metric, F.Cu at (245.9, 49.1)
- added C7: 47uF, Capacitor_SMD:C_0805_2012Metric, F.Cu at (171.7, 50.5)
- added C7: 47uF, Capacitor_SMD:C_0805_2012Metric, F.Cu at (219.7, 50.5)
- added C7: 47uF, Capacitor_SMD:C_0805_2012Metric, F.Cu at (243.7, 50.5)
- added C7: 47uF, Capacitor_SMD:C_0805_2012Metric, F.Cu at (291.7, 50.5)
- added C7: 47uF, Capacitor_SMD:C_0805_2012Metric, F.Cu at (195.7, 50.5)
- added C7: 47uF, Capacitor_SMD:C_0805_2012Metric, F.Cu at (267.7, 50.5)
- added C8: 10nF, Capacitor_SMD:C_0402_1005Metric, F.Cu at (229.4, 47.8)
- added C8: 10nF, Capacitor_SMD:C_0402_1005Metric, F.Cu at (277.4, 47.8)
- added C8: 10nF, Capacitor_SMD:C_0402_1005Metric, F.Cu at (181.4, 47.8)
- added C8: 10nF, Capacitor_SMD:C_0402_1005Metric, F.Cu at (253.4, 47.8)
- added C8: 10nF, Capacitor_SMD:C_0402_1005Metric, F.Cu at (157.4, 47.8)
- added C8: 10nF, Capacitor_SMD:C_0402_1005Metric, F.Cu at (205.4, 47.8)
- added C9: 10uF, Capacitor_SMD:C_0402_1005Metric, F.Cu at (156.3, 47.8)
- added C9: 10uF, Capacitor_SMD:C_0402_1005Metric, F.Cu at (276.3, 47.8)
- added C9: 10uF, Capacitor_SMD:C_0402_1005Metric, F.Cu at (252.3, 47.8)
- added C9: 10uF, Capacitor_SMD:C_0402_1005Metric, F.Cu at (228.3, 47.8)
- added C9: 10uF, Capacitor_SMD:C_0402_1005Metric, F.Cu at (204.3, 47.8)
- added C9: 10uF, Capacitor_SMD:C_0402_1005Metric, F.Cu at (180.3, 47.8)
- added D1: GREEN, CustomFootprints:LED0805-GREEN-RD, F.Cu at (196.5, 36.2)
- added D1: GREEN, CustomFootprints:LED0805-GREEN-RD, F.Cu at (220.5, 36.2)
- added D1: GREEN, CustomFootprints:LED0805-GREEN-RD, F.Cu at (292.5, 36.2)
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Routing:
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- added copper zone on F.Cu, net Board_5-/SensorCapV
- added copper zone on B.Cu, net Board_5-GND
- added copper zone on F.Cu, net Board_5-GND
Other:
- board size 132 x 147 mm -> 156 x 147 mm
- board text removed: "+"
- board text removed: "-"
